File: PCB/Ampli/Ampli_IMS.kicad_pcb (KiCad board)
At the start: 2 copper layers, 58.4 x 32 mm, 18 parts, among them J1 5227161-3, J2 5227161-3, J3 Conn_01x03_Male, P1 300K, U1 LMC6081, U2 LMC6081

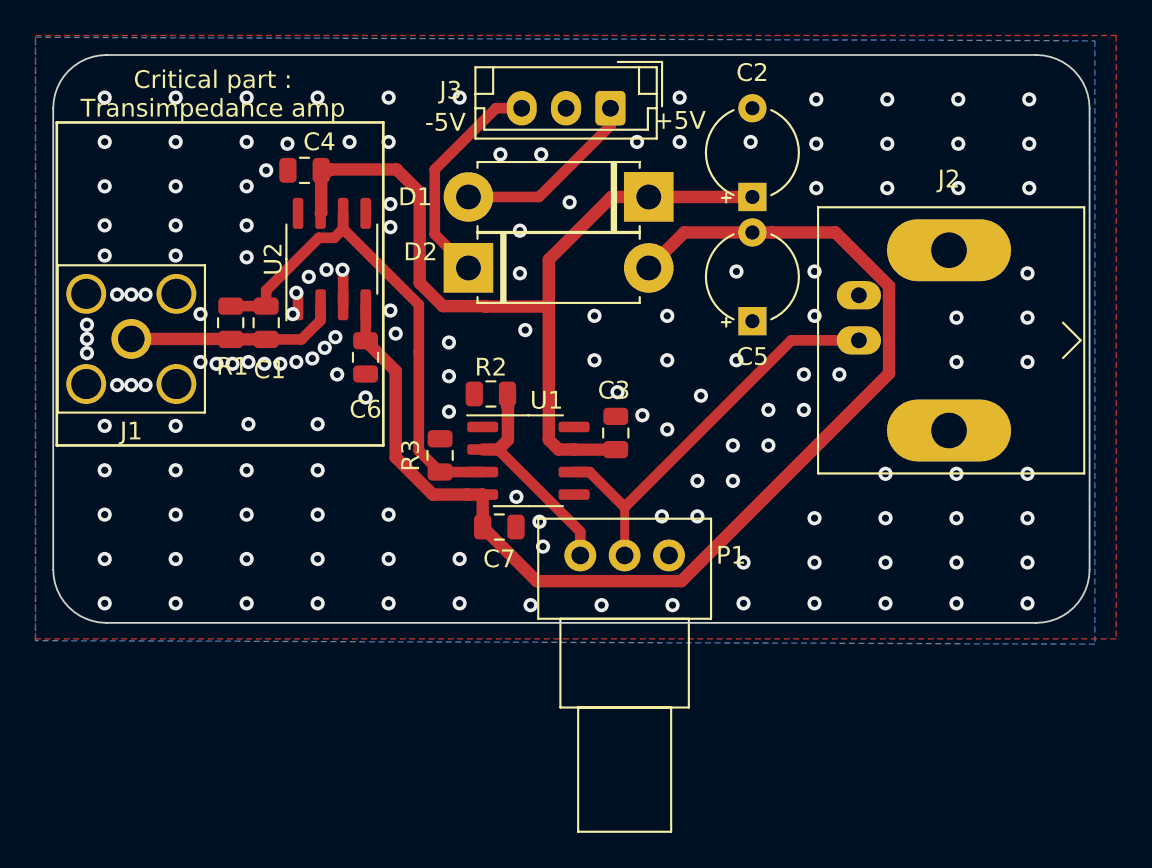
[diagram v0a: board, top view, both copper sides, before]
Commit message: GND guards are neat!
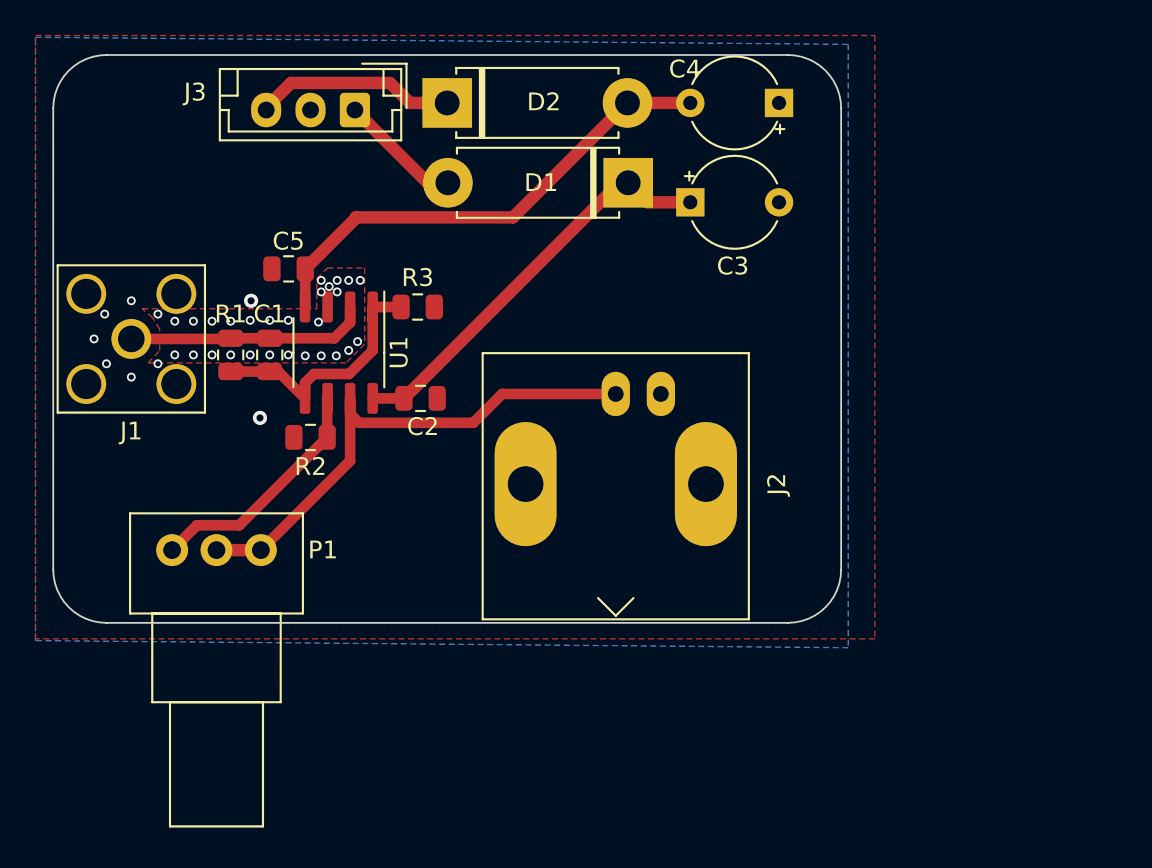
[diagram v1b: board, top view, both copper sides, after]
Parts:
- removed C6, C7: 0.1uF, Capacitor_SMD:C_0805_2012Metric
- removed U2: LMC6081, Package_SO:SO-8_3.9x4.9mm_P1.27mm
- C2, C5: value 47uF Tant -> 0.1uF; footprint Capacitor_THT:CP_Radial_Tantal_D5.0mm_P5.00mm -> Capacitor_SMD:C_0805_2012Metric
- C3, C4: value 0.1uF -> 47uF Tant; footprint Capacitor_SMD:C_0805_2012Metric -> Capacitor_THT:CP_Radial_Tantal_D5.0mm_P5.00mm
- U1: value LMC6081 -> LMC6082
- moved C4 27.0 mm to (65.5, 20.7)
- moved C5 26.3 mm to (37.9, 30.1), turned to 180 degrees
- moved P1 23.0 mm to (31.3, 45.9)
- moved C2 21.9 mm to (45.3, 37.4), turned to 0 degrees
- moved J3 14.4 mm to (41.6, 21.1)
- moved J2 14.0 mm to (56.3, 37.1), turned to 180 degrees
- moved C3 13.7 mm to (60.5, 26.3), turned to 0 degrees
- moved U1 12.3 mm to (40.7, 34.8), turned to 270 degrees
- moved R2 10.5 mm to (39.1, 39.5)
- moved D2 9.38 mm to (46.8, 20.7)
- moved R3 8.46 mm to (45.1, 32.2), turned to 0 degrees
- moved C1 1.82 mm to (36.8, 34.9), turned to 90 degrees
- moved R1 1.81 mm to (34.6, 34.9), turned to 90 degrees
- moved D1 1.41 mm to (57.0, 25.2)
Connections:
- C4 pad 1: /+5V -> GND
- C4 pad 2: GND -> /-5V
- C5 pad 1: GND -> /-5V
- C5 pad 2: /-5V -> GND
- P1 pad 3: Net-(P1-Pad3) -> Net-(J2-Pad1)
- U1 pad 1: (no net) -> Net-(C1-Pad1)
- U1 pad 2: Net-(P1-Pad1) -> Net-(C1-Pad2)
- U1 pad 3: Net-(C1-Pad1) -> GND
- U1 pad 5: (no net) -> Net-(C1-Pad1)
- U1 pad 6: Net-(J2-Pad1) -> Net-(P1-Pad1)
- U1 pad 7: /+5V -> Net-(J2-Pad1)
- U1 pad 8: (no net) -> /+5V
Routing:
- net /-5V: track 66.5 -> 27.8 mm
- net /+5V: track 48.6 -> 23.4 mm
- net Net-(C1-Pad1): track 27.9 -> 15.1 mm
- net Net-(J2-Pad1): track 23.5 -> 29.9 mm
- net Net-(D1-Pad2): track 10.6 -> 6.94 mm
- net GND: track 2.04 -> 0.00 mm, vias 153 -> 36
- net Net-(C1-Pad2): track 12.0 -> 13.6 mm
- net Net-(P1-Pad1): track 12.1 -> 13.6 mm
- net Net-(D2-Pad1): track 12.7 -> 11.4 mm
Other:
- board size 58.4 x 32 mm -> 44.4 x 32 mm
- board text removed: "+5V"
- board text removed: "-5V"
- board text removed: "Critical part : Transimpedance amp"
